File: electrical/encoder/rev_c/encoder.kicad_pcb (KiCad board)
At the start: 2 copper layers, 14.8 x 48 mm, 5 parts, among them CN1 ENCODER;2xM1x3RA, Q1 AH1806;SC59, Q2 AH1806;SC59

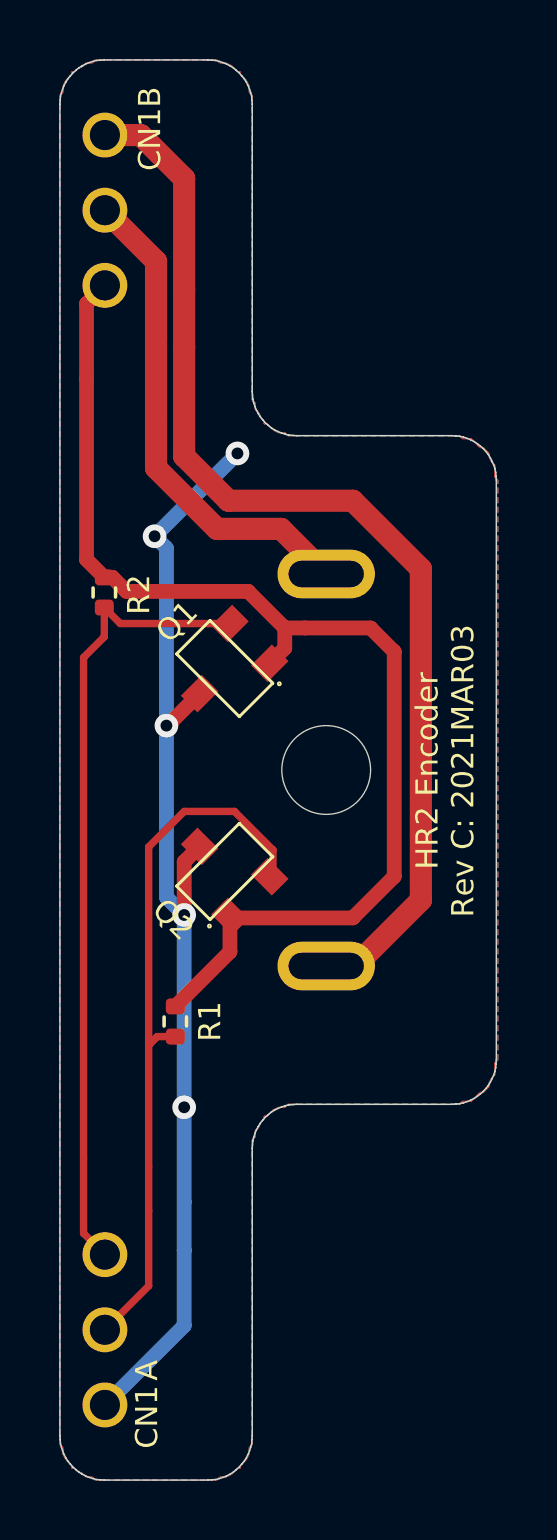
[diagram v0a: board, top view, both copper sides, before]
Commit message: Wrapped up Encoder Rev. C.
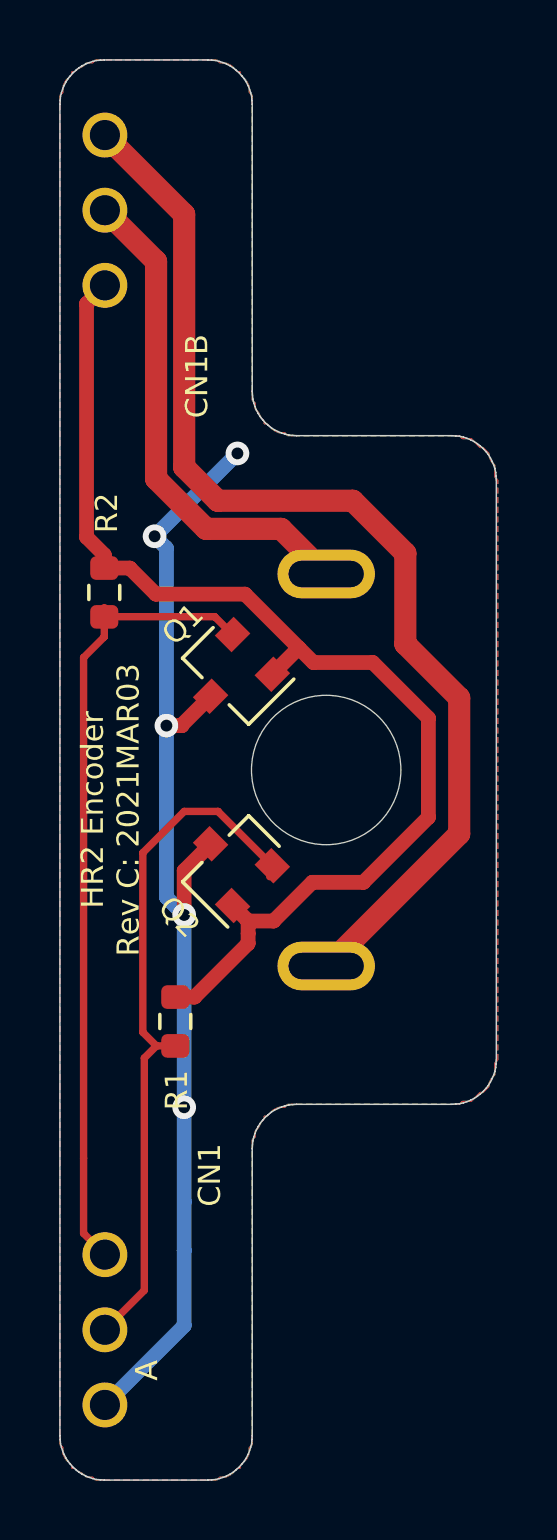
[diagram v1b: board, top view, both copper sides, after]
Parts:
- Q1, Q2: value AH1806;SC59 -> DRV5013FAQDBZR;SOT23; footprint HR2:SC59 -> Package_TO_SOT_SMD:SOT-23
- R1, R2: value 100Ω;1005 -> 47KΩ;1608; footprint Resistor_SMD:R_0402_1005Metric -> Resistor_SMD:R_0603_1608Metric
- moved Q1 0.33 mm to (96.8, 96.8), turned to 225 degrees
- moved Q2 0.33 mm to (96.8, 103.2), turned to 135 degrees
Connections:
- Q1 pad 2: /GND -> /QUADB
- Q1 pad 3: /QUADB -> /GND
- Q2 pad 2: /GND -> /QUADA
- Q2 pad 3: /QUADA -> /GND
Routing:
- net /QUADA: track 24.2 -> 23.5 mm
- net /GND: track 38.9 -> 39.5 mm
